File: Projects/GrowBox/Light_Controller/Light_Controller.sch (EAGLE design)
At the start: 12 parts, among them Q1 BC847BSMD, Q2 BC847BSMD, Q3 BC847BSMD, Q4 BC847BSMD

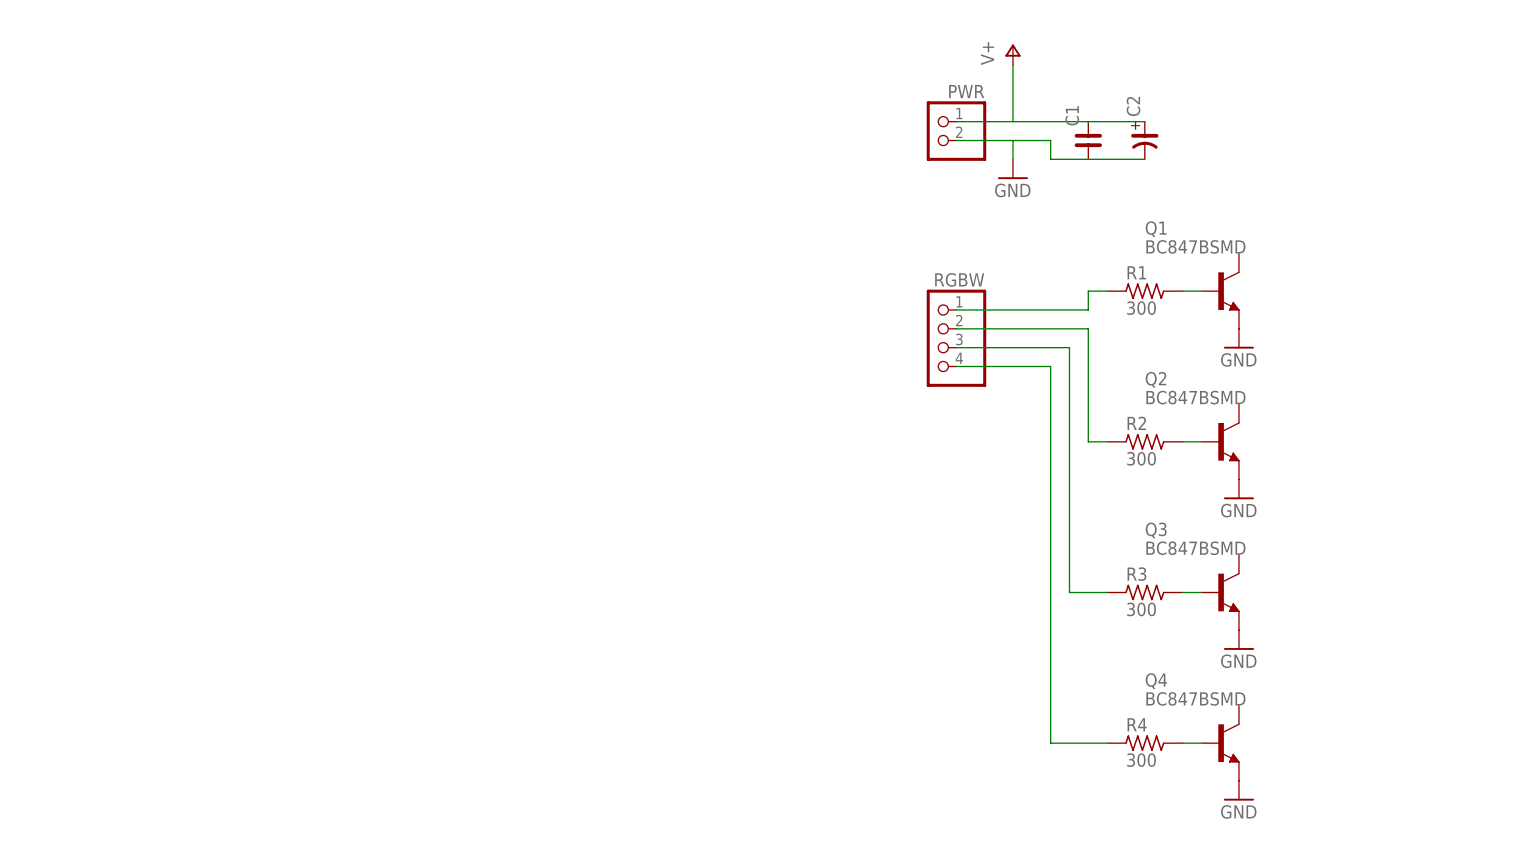
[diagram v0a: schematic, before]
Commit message: Added projects from work...
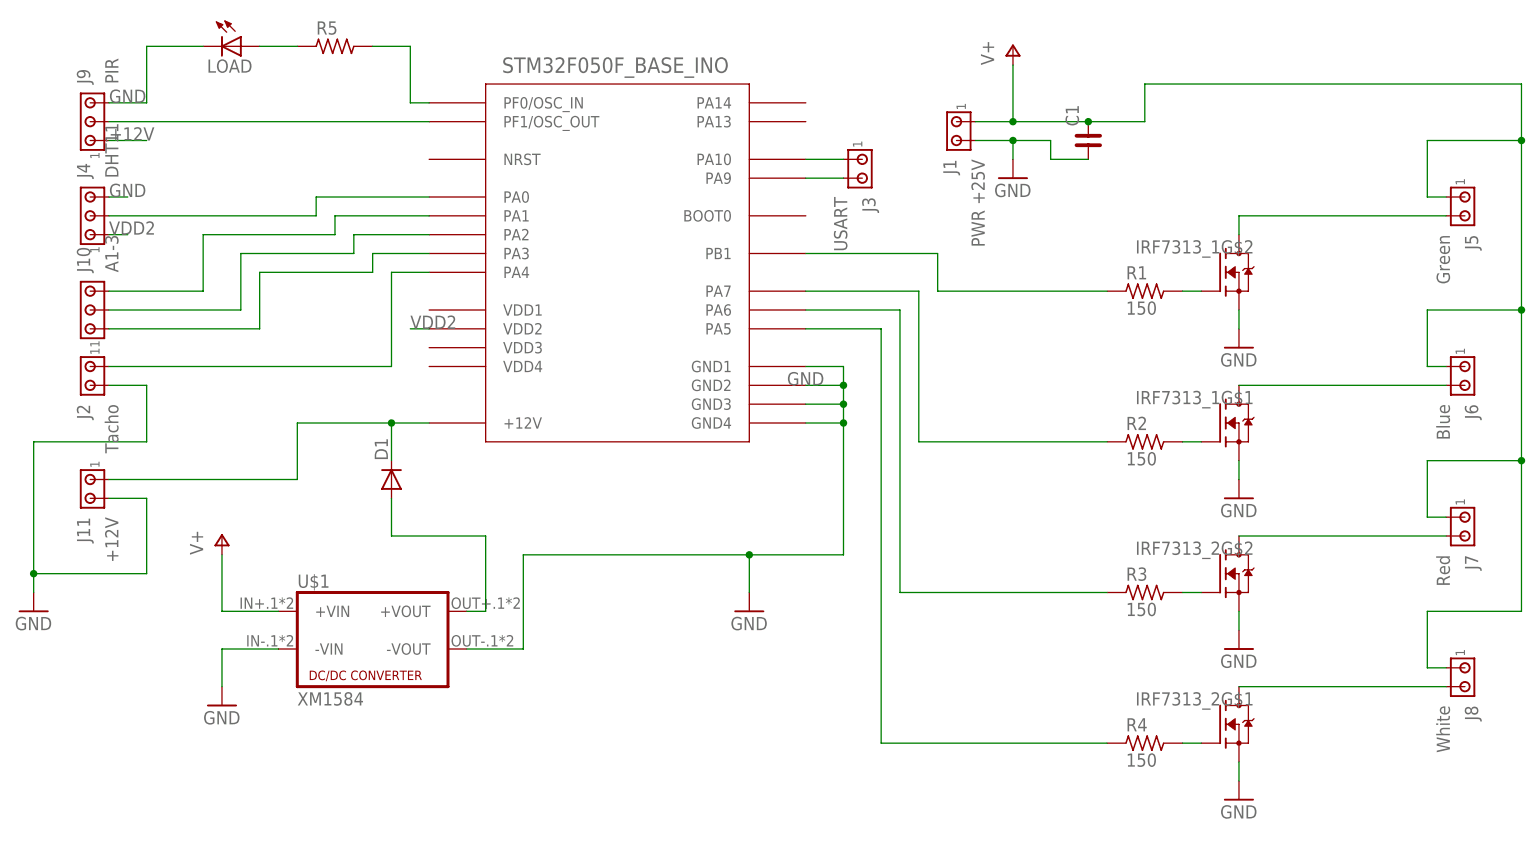
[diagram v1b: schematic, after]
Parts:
- removed C2: (no value), rc-master-smd:CP_SV-D
- removed PWR: (no value), pinhead-2:PINHD-1X02_2.54-S
- removed Q1, Q2, Q3, Q4: BC847BSMD, transistor-npn:BC847BSMD
- removed RGBW: (no value), pinhead-2:PINHD-1X04_2.54-S
- added D1: (no value), diode:DIODE-DO214AC
- added IRF7313_1, IRF7313_2: IRF7313, my-library:IRF7313
- added J1: PWR +25V, con-amp:MTA02-100
- added J10: A1-3, con-amp:MTA03-100
- added J11: +12V, con-amp:MTA02-100
- added J2: Tacho, con-amp:MTA02-100
- added J3: USART, con-amp:MTA02-100
- added J4: DHT11, con-amp:MTA03-100
- added J5: Green, con-amp:MTA02-100
- added J6: Blue, con-amp:MTA02-100
- added J7: Red, con-amp:MTA02-100
- added J8: White, con-amp:MTA02-100
- added J9: PIR, con-amp:MTA03-100
- added LOAD: (no value), led:LEDCHIPLED_1206
- added R5: (no value), rc-master-smd:R_1206
- added STM321: STM32F050F_BASE_INO, my-library:STM32F050F_BASE_INO
- added U$1: XM1584, my-library:XM1584
- R1, R2, R3, R4: value 300 -> 150
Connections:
- new net +12V: D1.C, J11.1, J9.1, STM321.+12V
- new net N$10: R2.1, STM321.PA7
- new net N$11: LOAD.A, R5.1
- new net N$12: IRF7313_1G$1.D, J6.2
- new net N$13: J3.1, STM321.PA10
- new net N$14: IRF7313_2G$2.D, J7.2
- new net N$15: J3.2, STM321.PA9
- new net N$16: R5.2, STM321.PF0/OSC_IN
- new net N$17: J4.2, STM321.PA0
- new net N$18: J9.2, STM321.PF1/OSC_OUT
- new net N$19: IRF7313_2G$1.D, J8.2
- new net N$20: J10.3, STM321.PA1
- new net N$21: J10.2, STM321.PA2
- new net N$22: J10.1, STM321.PA3
- new net N$23: D1.A, U$1.+VOUT
- new net N$9: R3.1, STM321.PA6
- new net VDD2: J4.1, STM321.VDD2
- net GND: now also IRF7313_1G$1.S, IRF7313_1G$2.S, IRF7313_2G$1.S, IRF7313_2G$2.S, J1.2, J11.2, J2.2, J4.3, J9.3, LOAD.C, STM321.GND1, STM321.GND2, STM321.GND3, STM321.GND4, U$1.-VIN, U$1.-VOUT; no longer C2.-, PWR.2, Q1.E, Q2.E, Q3.E, Q4.E
- net N$1: now also STM321.PB1; no longer RGBW.1
- net N$2: now also IRF7313_1G$2.D, J5.2; no longer R2.1, RGBW.2
- net N$3: now also J2.1, STM321.PA4; no longer R3.1, RGBW.3
- net N$4: now also STM321.PA5; no longer RGBW.4
- net N$5: now also IRF7313_1G$2.G; no longer Q1.B
- net N$6: now also IRF7313_1G$1.G; no longer Q2.B
- net N$7: now also IRF7313_2G$1.G, R4.2; no longer Q3.B, R3.2
- net N$8: now also IRF7313_2G$2.G, R3.2; no longer Q4.B, R4.2
- net V+: now also J1.1, J5.1, J6.1, J7.1, J8.1, U$1.+VIN; no longer C2.+, PWR.1
